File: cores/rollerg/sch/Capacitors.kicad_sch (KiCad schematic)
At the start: 1 part

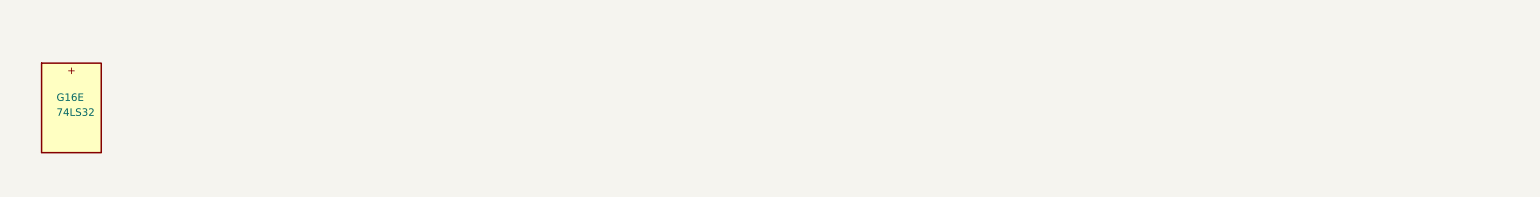
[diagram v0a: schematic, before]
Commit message: almost complete rollerg sch
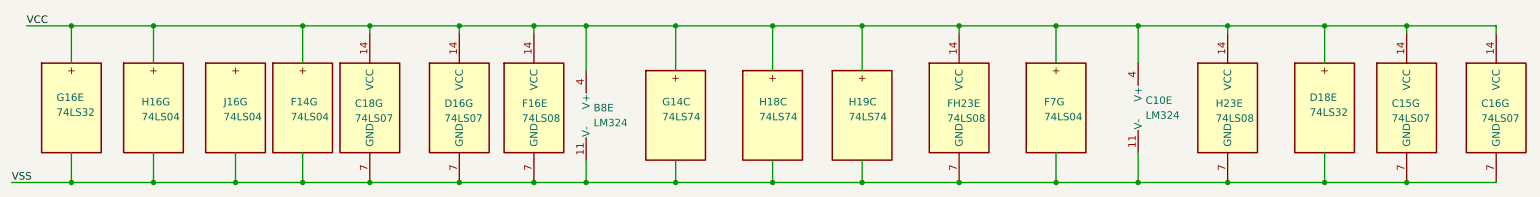
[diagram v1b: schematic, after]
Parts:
- added B8, C10: LM324, symbol Amplifier_Operational:LM324
- added C15, C16, C18, D16: 74LS07, symbol 74xx:74LS07
- added D18: 74LS32, symbol jt74:74LS32
- added F14, F7, H16, J16: 74LS04, symbol jt74:74LS04
- added F16, FH23, H23: 74LS08, symbol 74xx:74LS08
- added G14, H18, H19: 74LS74, symbol jt74:74LS74
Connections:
- net GND: now also B8.11 (V-), C10.11 (V-), C15.7 (GND), C16.7 (GND), C18.7 (GND), D16.7 (GND), D18.7 (GND), F14.7 (GND), F16.7 (GND), F7.7 (GND), FH23.7 (GND), G14.7 (GND), H16.7 (GND), H18.7 (GND), H19.7 (GND), H23.7 (GND), J16.7 (GND)
- net VCC: now also B8.4 (V+), C10.4 (V+), C15.14 (VCC), C16.14 (VCC), C18.14 (VCC), D16.14 (VCC), D18.14 (VCC), F14.14 (VCC), F16.14 (VCC), F7.14 (VCC), FH23.14 (VCC), G14.14 (VCC), H16.14 (VCC), H18.14 (VCC), H19.14 (VCC), H23.14 (VCC), J16.14 (VCC)
